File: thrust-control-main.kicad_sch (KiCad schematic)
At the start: 18 parts, among them U20 MCP3208, U21 LTC2620IGN, U33 LM358, U34 LM358, U45 MAX6103, U46 LM358, U62 LM358

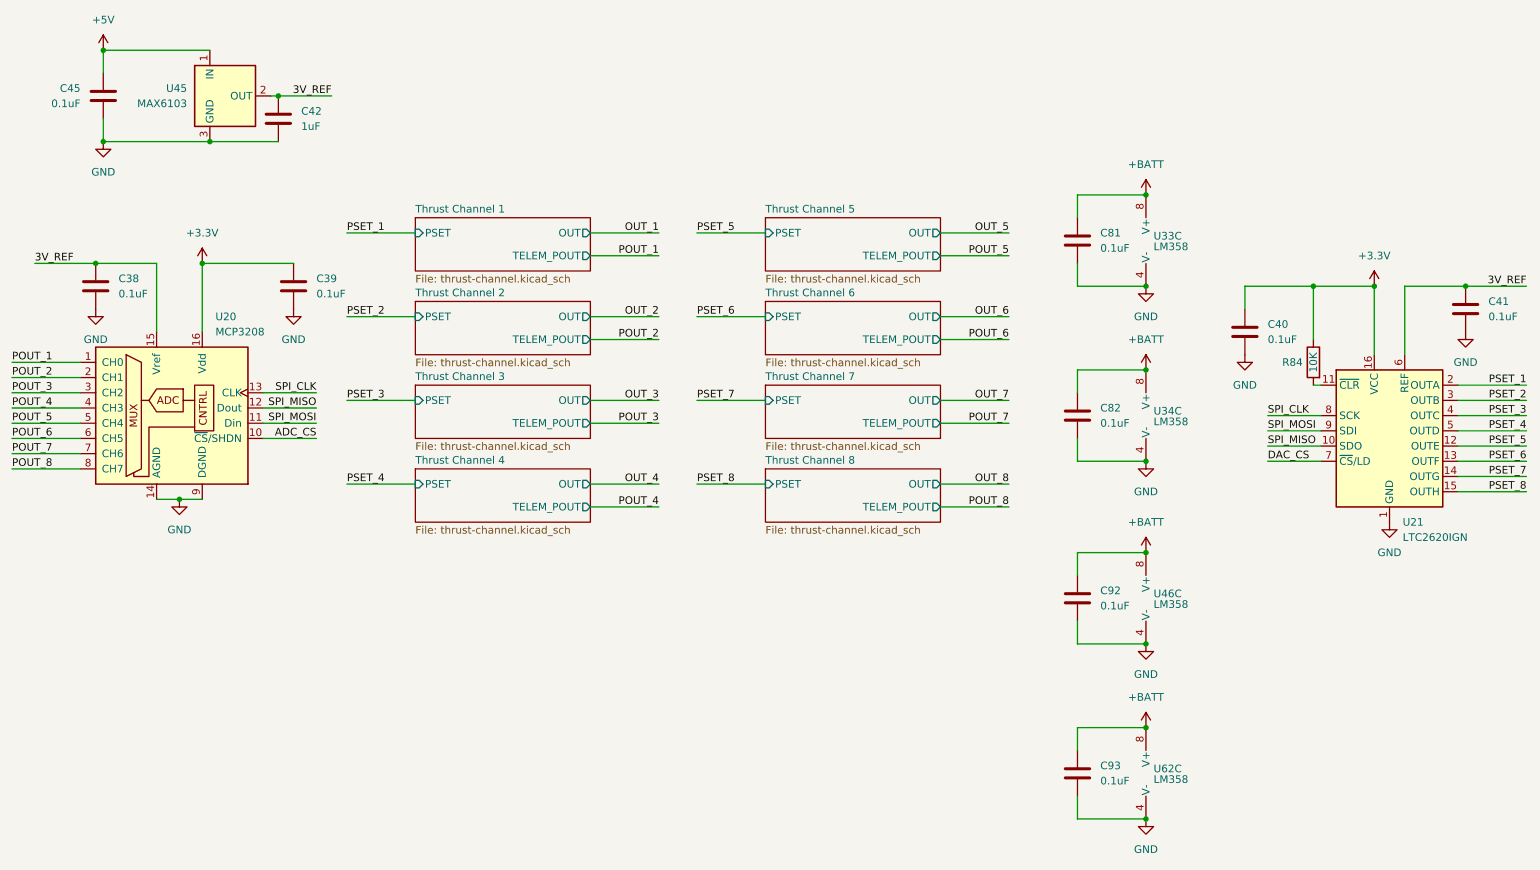
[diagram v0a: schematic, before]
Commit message: work
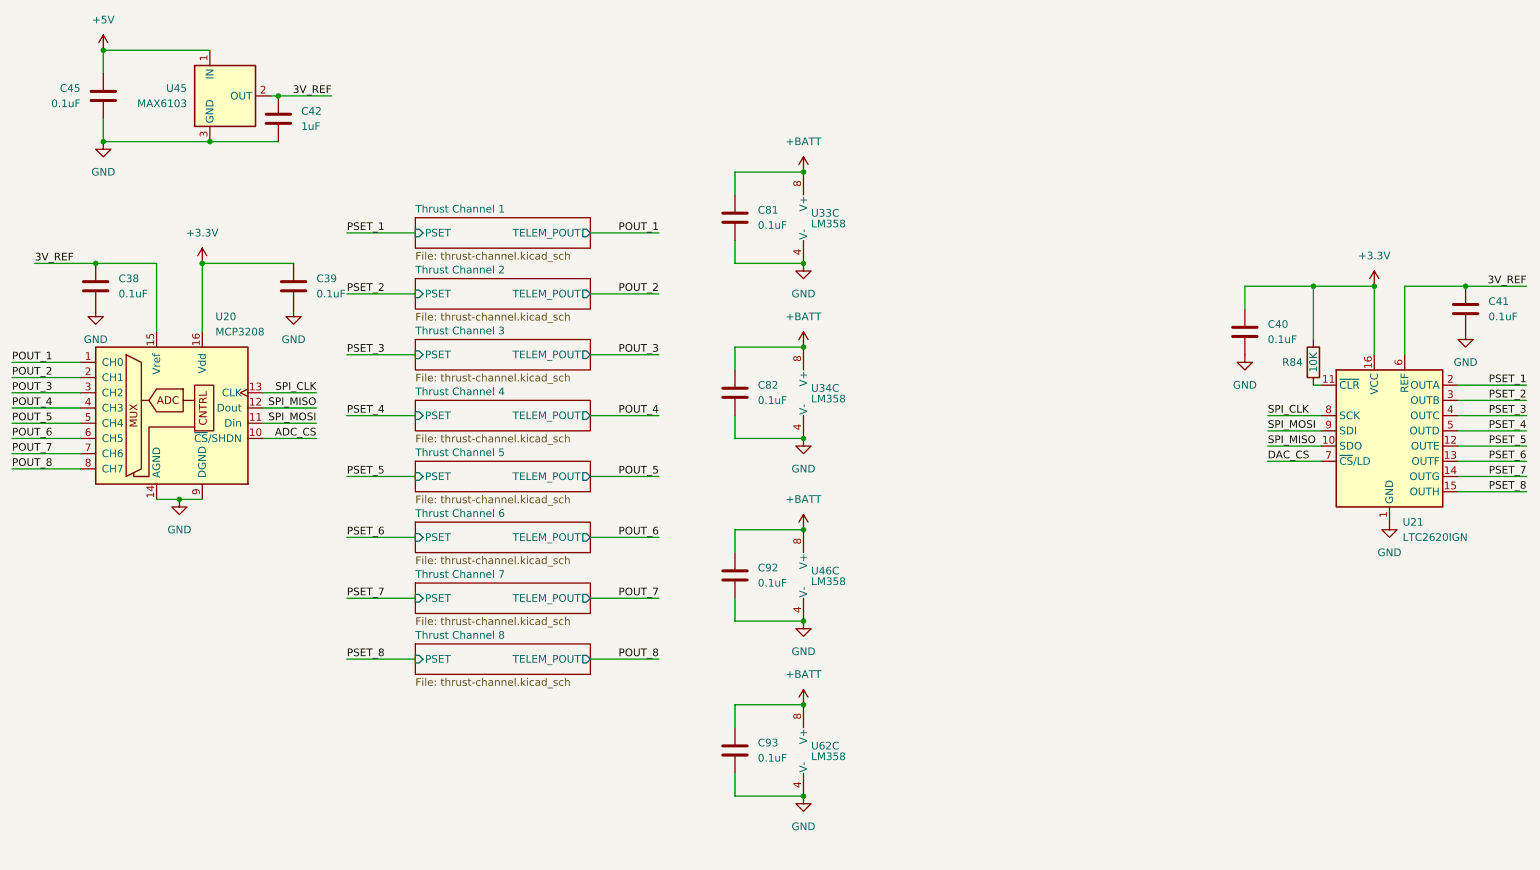
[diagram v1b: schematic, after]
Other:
- sheet Thrust Channel 1 ports: added none; removed OUT
- sheet Thrust Channel 2 ports: added none; removed OUT
- sheet Thrust Channel 3 ports: added none; removed OUT
- sheet Thrust Channel 4 ports: added none; removed OUT
- sheet Thrust Channel 5 ports: added none; removed OUT
- sheet Thrust Channel 6 ports: added none; removed OUT
- sheet Thrust Channel 7 ports: added none; removed OUT
- sheet Thrust Channel 8 ports: added none; removed OUT
- moved on the sheet: C81, C82, C92, C93, U33C, U34C, U46C, U62C
